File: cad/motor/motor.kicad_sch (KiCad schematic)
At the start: 25 parts, among them Q1 NMOS, Q10 PMOS, Q11 NMOS, Q12 NMOS, Q13 PMOS, Q14 PMOS, Q2 NMOS, Q3 PMOS, Q4 PMOS, Q5 NMOS, Q6 PMOS, Q7 PMOS, Q8 PMOS, Q9 NMOS

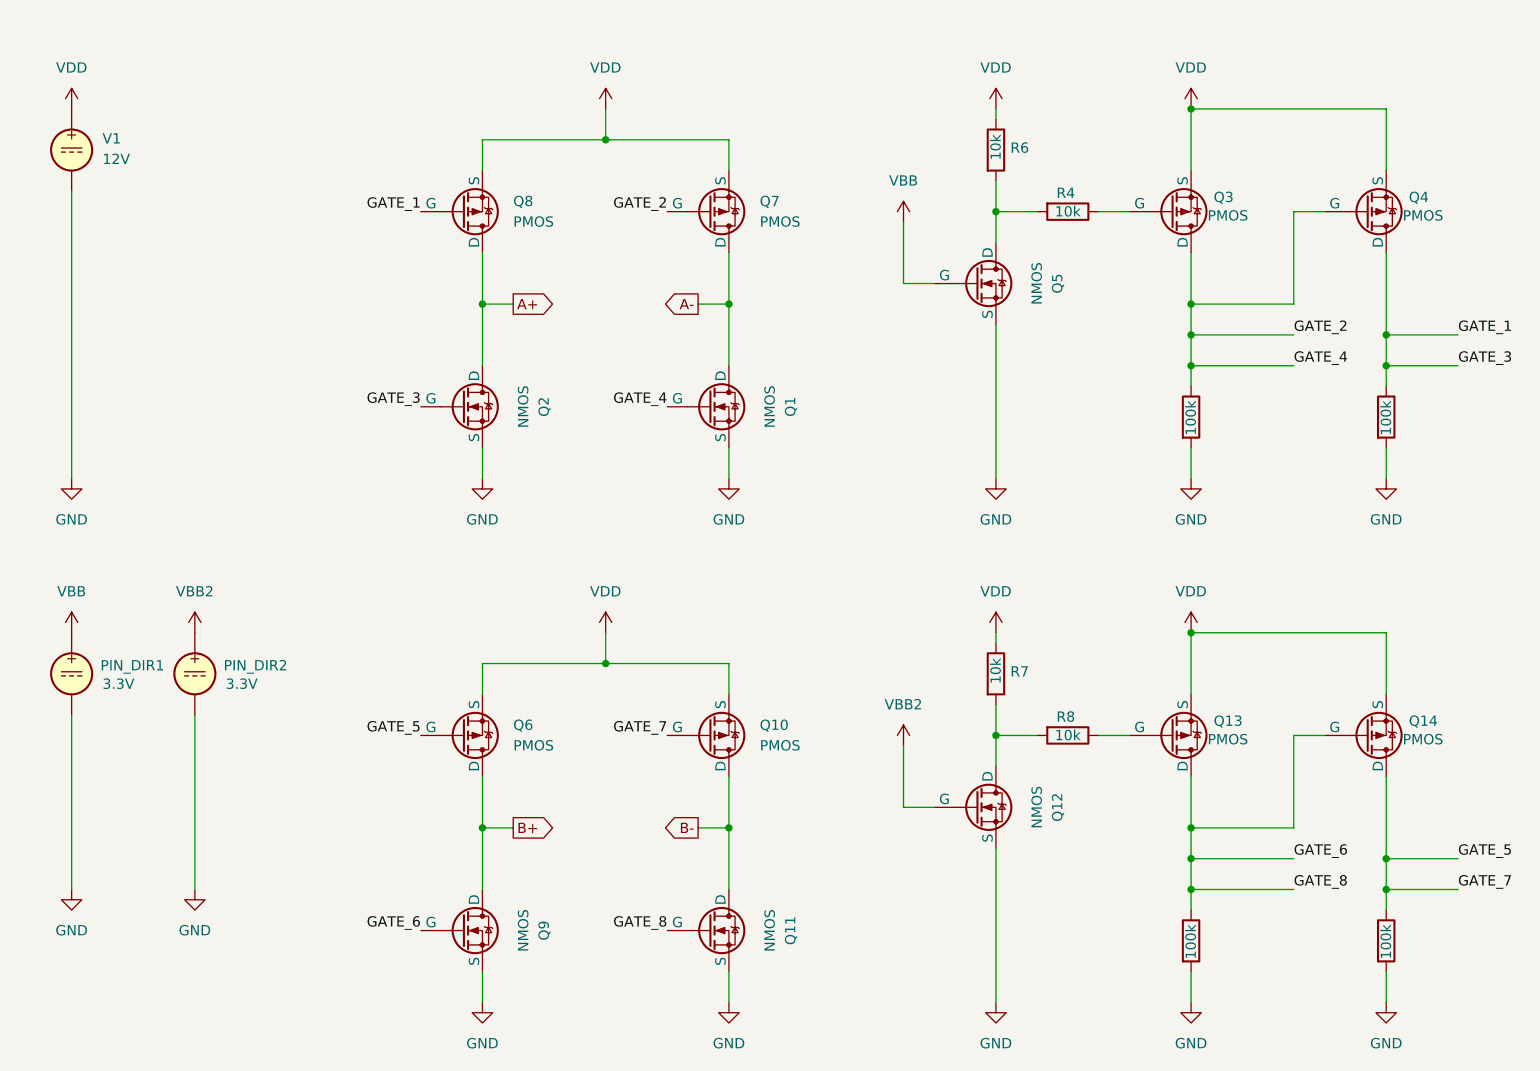
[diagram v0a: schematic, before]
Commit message: more cad
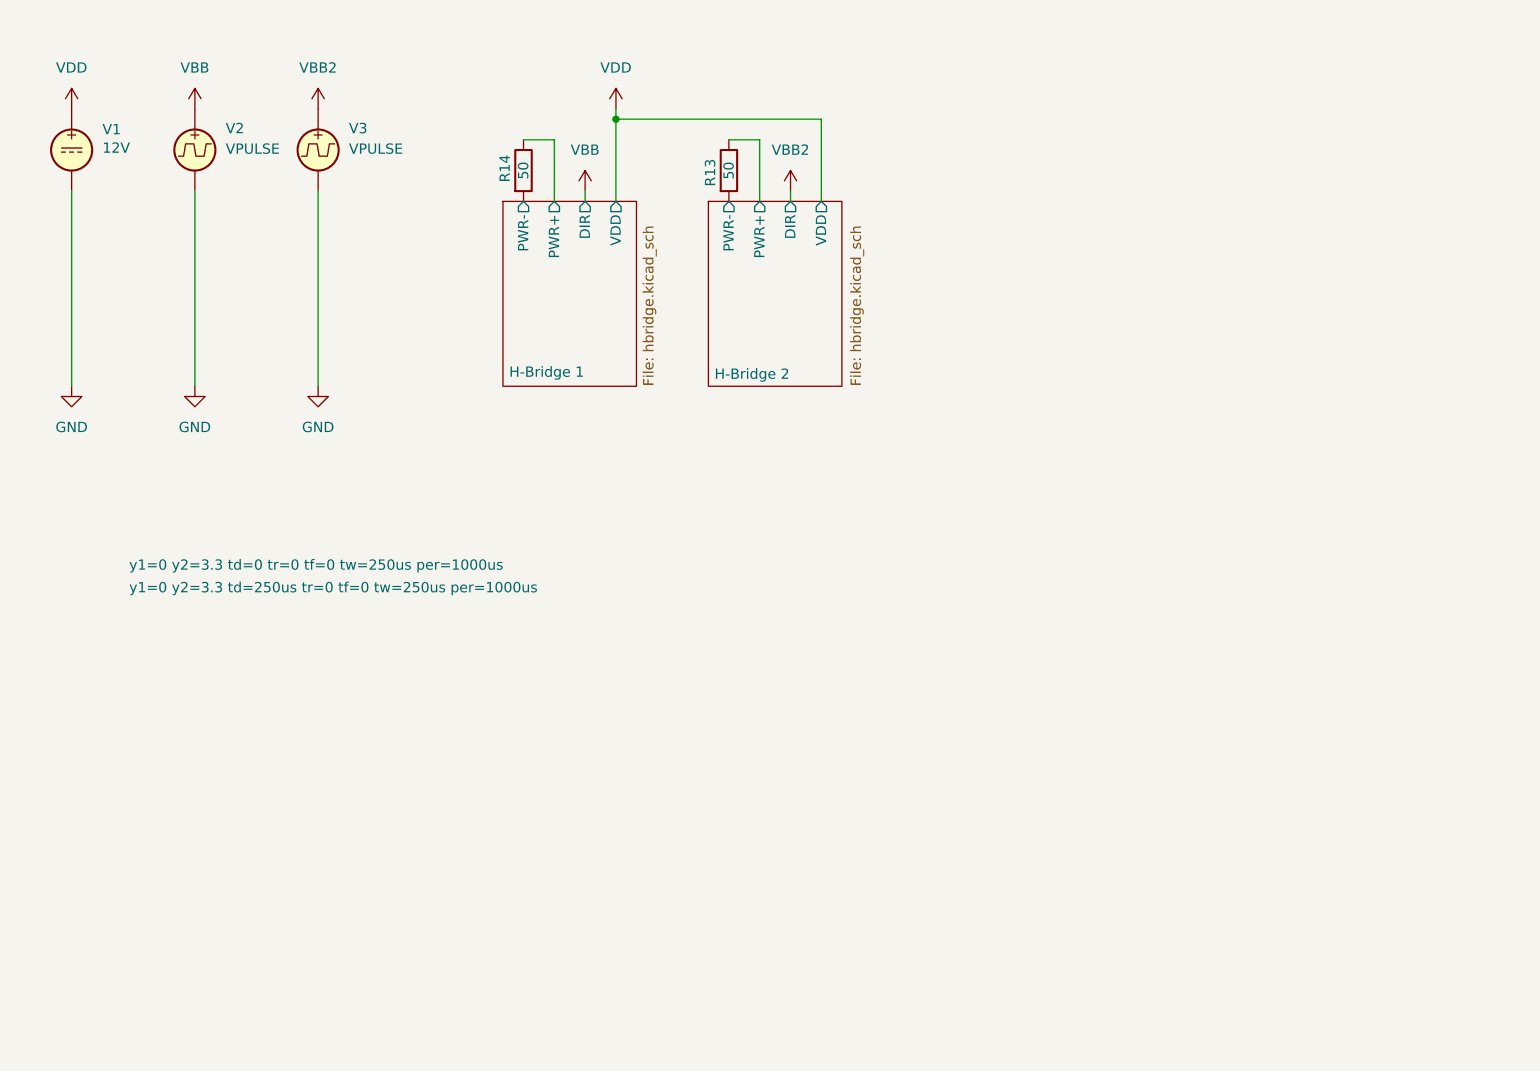
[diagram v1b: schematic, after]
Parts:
- removed PIN_DIR1, PIN_DIR2: 3.3V, symbol Simulation_SPICE:VDC
- removed Q1, Q11, Q12, Q2, Q5, Q9: NMOS, symbol Simulation_SPICE:NMOS
- removed Q10, Q13, Q14, Q3, Q4, Q6, Q7, Q8: PMOS, symbol Simulation_SPICE:PMOS
- removed R10, R2, R5, R9: 100k, symbol Device:R
- removed R4, R6, R7, R8: 10k, symbol Device:R
- added R13, R14: 50, symbol Device:R
- added V2, V3: VPULSE, symbol Simulation_SPICE:VPULSE
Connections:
- net GND: now also V2.2, V3.2
- net VBB: now also V2.1
- net VBB2: now also V3.1
- new net H-Bridge 1/PWR+: R14.1
- new net H-Bridge 1/PWR-: R14.2
- new net H-Bridge 2/PWR+: R13.1
- new net H-Bridge 2/PWR-: R13.2
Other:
- added sheet H-Bridge 1 (hbridge.kicad_sch)
- added sheet H-Bridge 2 (hbridge.kicad_sch)

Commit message: enable/disable
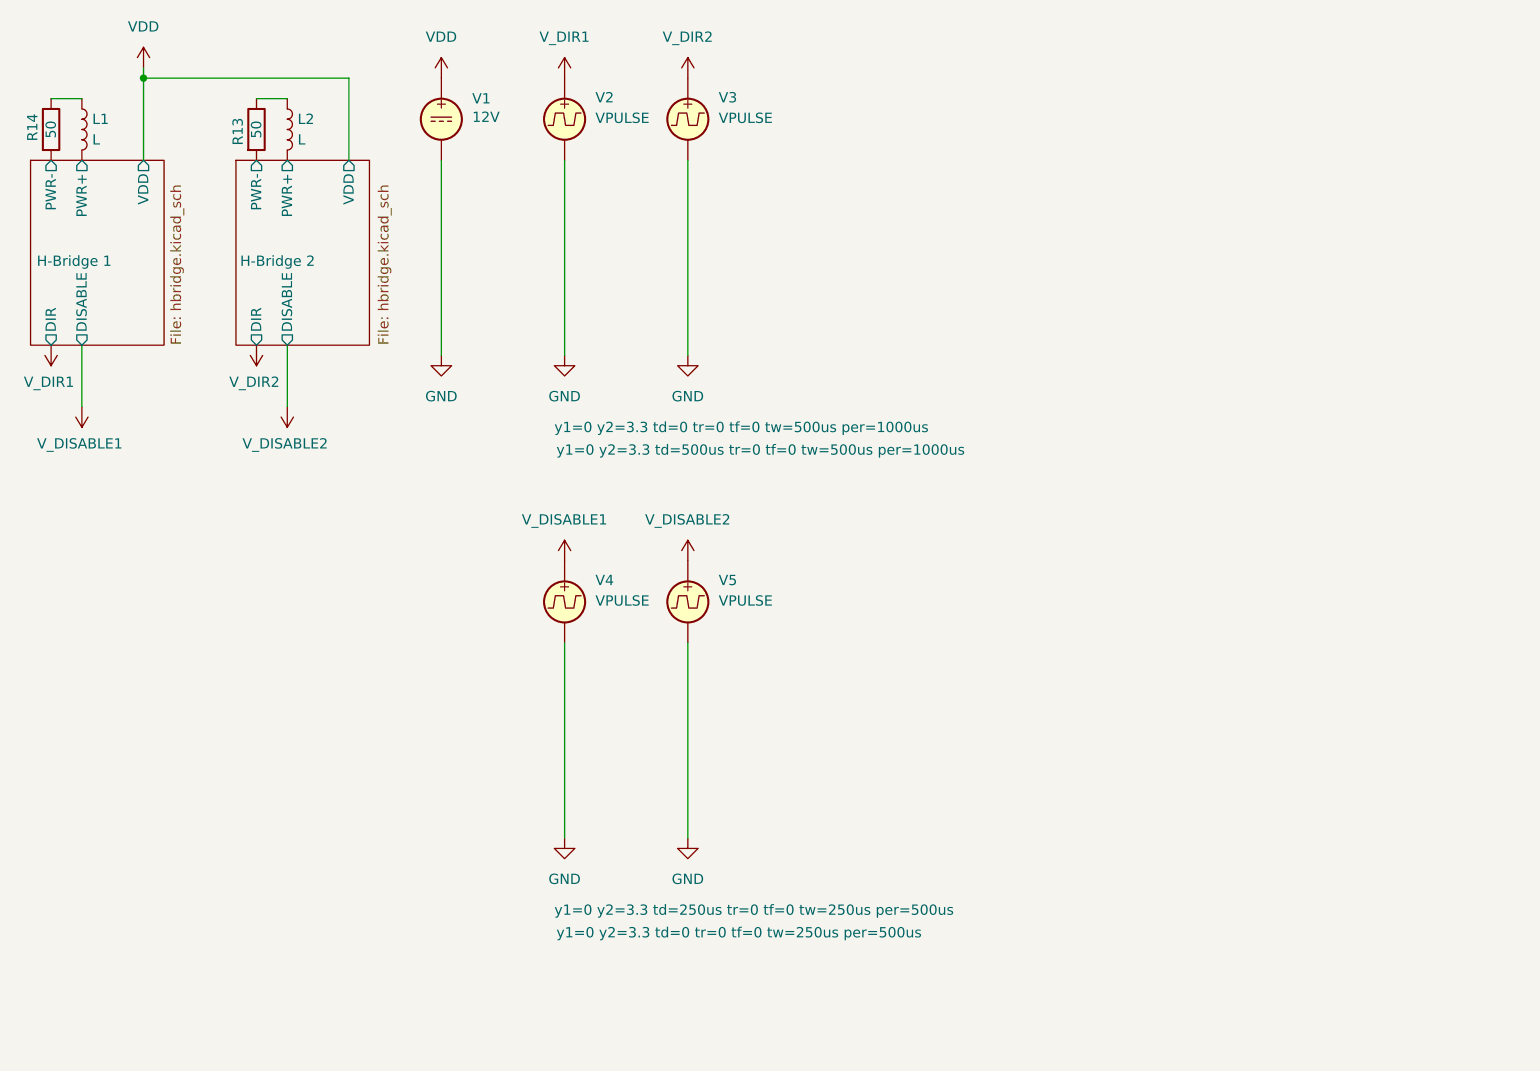
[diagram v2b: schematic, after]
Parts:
- added L1, L2: L, symbol Device:L
- added V4, V5: VPULSE, symbol Simulation_SPICE:VPULSE
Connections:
- net GND: now also V4.2, V5.2
- net H-Bridge 1/PWR+: now also L1.2; no longer R14.1
- net H-Bridge 2/PWR+: now also L2.2; no longer R13.1
- net VBB renamed V_DIR1
- net VBB2 renamed V_DIR2
- new net: L1.1, R14.1
- new net: L2.1, R13.1
- new net V_DISABLE1: V4.1
- new net V_DISABLE2: V5.1
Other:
- sheet H-Bridge 1 ports: added DISABLE; removed none
- sheet H-Bridge 2 ports: added DISABLE; removed none
- moved on the sheet: R13, R14, V1, V2, V3
